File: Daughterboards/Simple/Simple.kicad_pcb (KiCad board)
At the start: 2 copper layers, 54 x 36 mm, 29 parts, among them J1 I2C EXT, J2 HRO-TYPEC-M12, J3 BATTERY JST, J6 FFC, J7 DEBUG, M1 M.2_Key_E, U1 SRV05-4, U4 XC6206P332MR

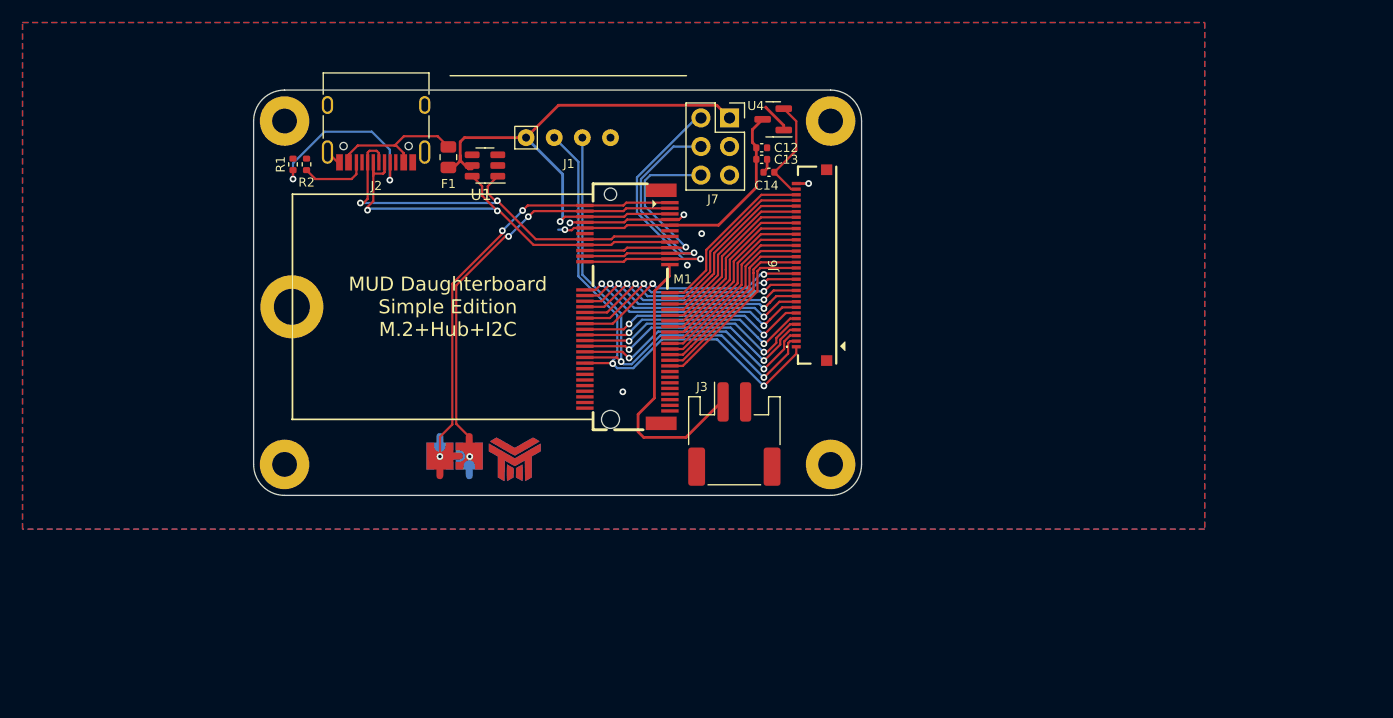
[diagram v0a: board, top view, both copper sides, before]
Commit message: prettify files a lil bit
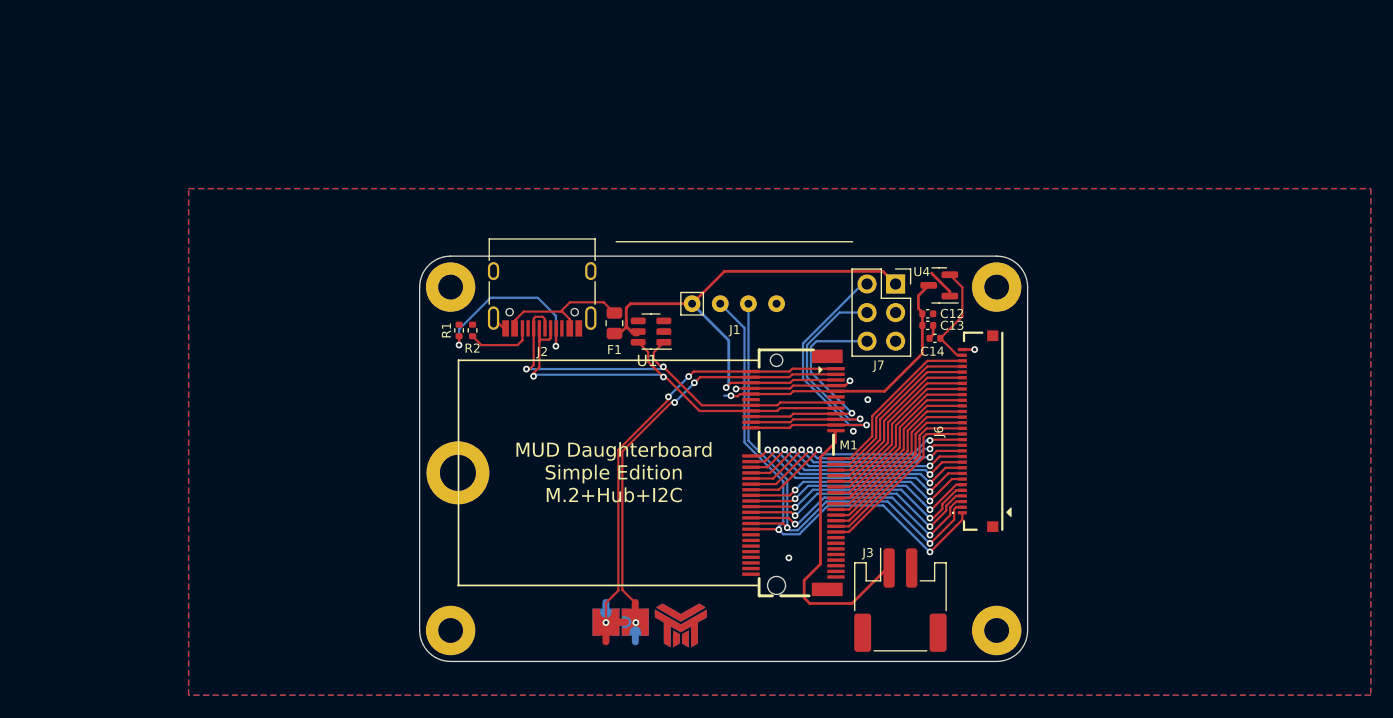
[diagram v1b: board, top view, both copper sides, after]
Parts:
- moved C12 20.9 mm to (59.9, 19.9)
- moved C13 20.9 mm to (59.9, 20.9)
- moved C14 20.9 mm to (60.5, 22.1)
- moved H1 20.9 mm to (17.5, 17.5)
- moved H2 20.9 mm to (66.0, 48.0)
- moved H3 20.9 mm to (66.0, 17.5)
- moved H4 20.9 mm to (17.5, 48.0)
- moved H5 20.9 mm to (18.1, 34.0)
- moved J1 20.9 mm to (42.7, 13.5)
- moved J7 20.9 mm to (57.0, 17.2)
- moved LO1 20.9 mm to (38.0, 47.5)
- moved LO2 20.9 mm to (32.6, 47.2)
- moved LO3 20.9 mm to (32.6, 47.2)
- moved LO4 20.9 mm to (38.0, 47.5)
- moved M1 20.9 mm to (48.0, 34.0)
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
